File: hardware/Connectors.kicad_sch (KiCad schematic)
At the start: 4 parts, among them J2 Conn_02x20_Odd_Even, J3 M80-8420445, U1 AS222-35PN-933

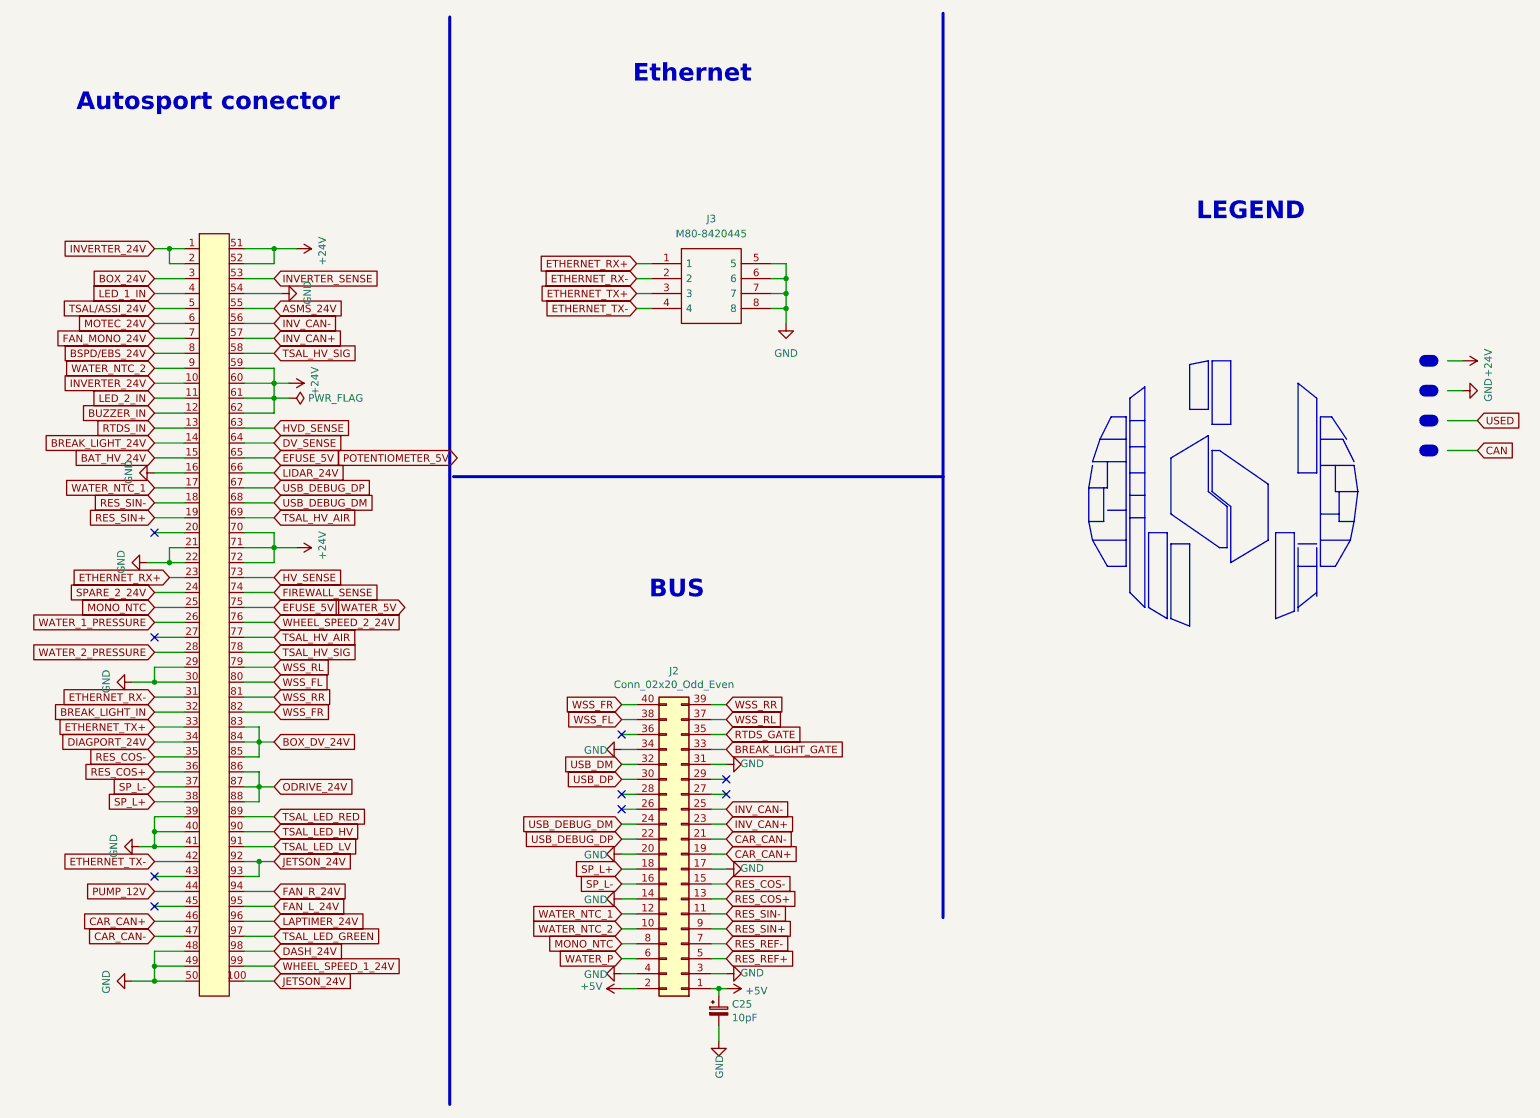
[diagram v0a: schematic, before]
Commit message: changed some footprints for clarity, and made some progress on board
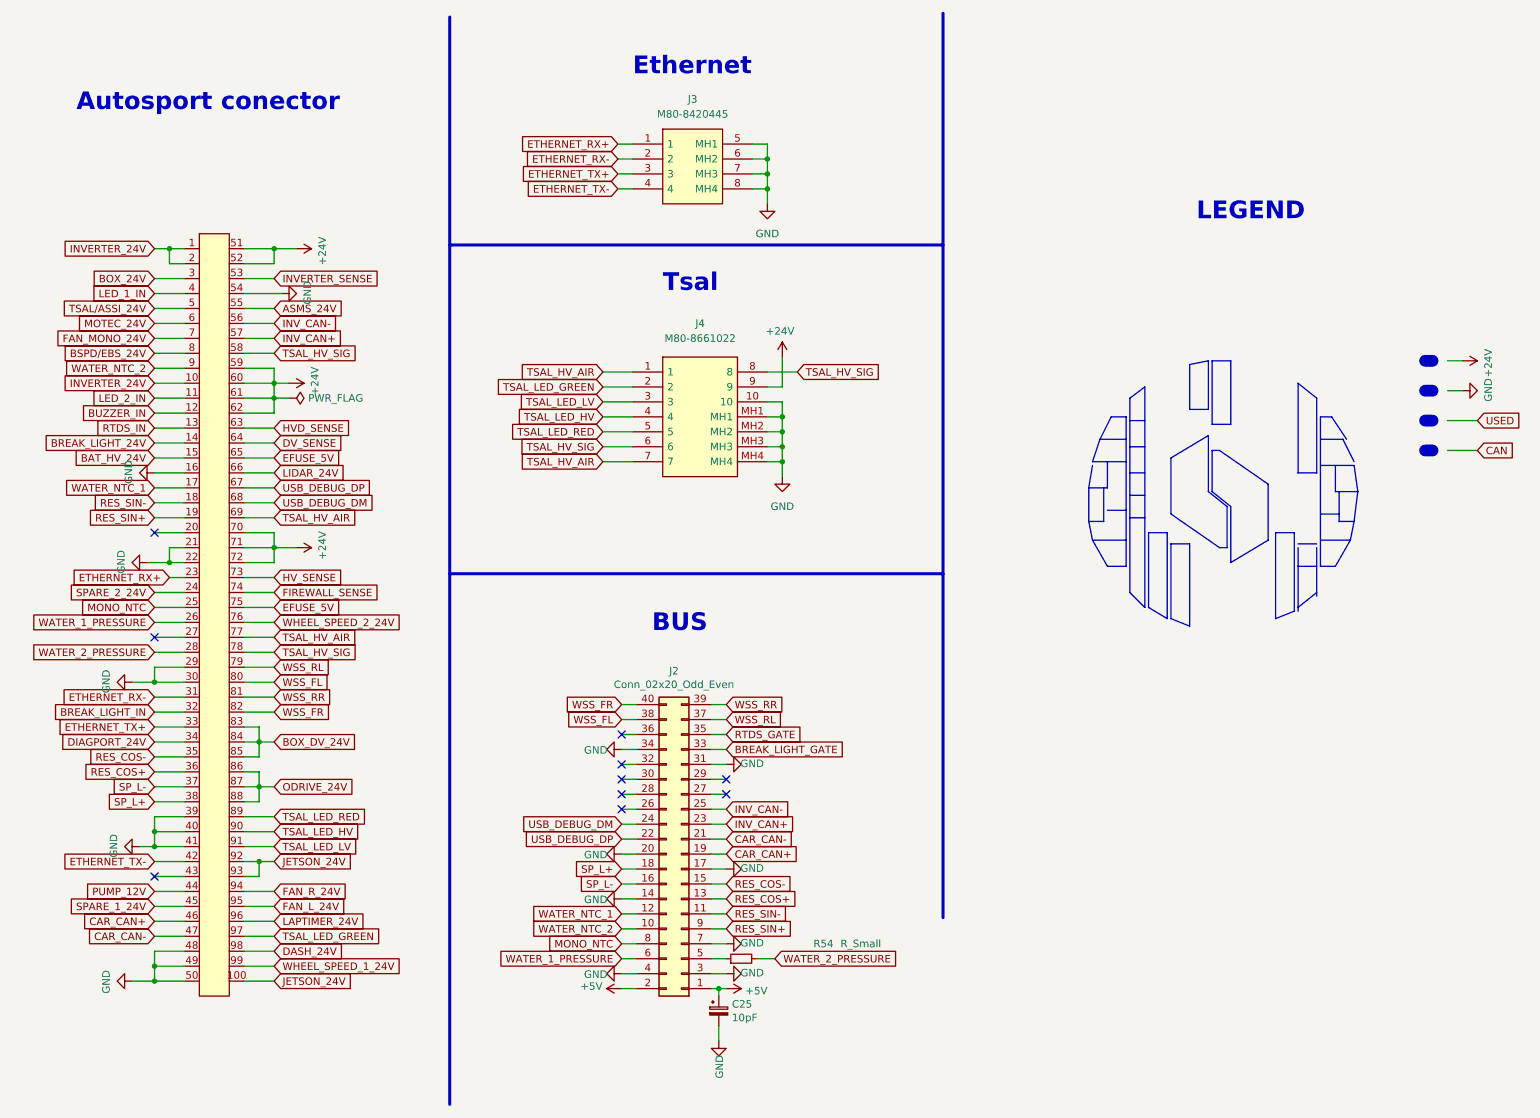
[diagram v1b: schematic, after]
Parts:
- added J4: M80-8661022, M80-8661022:M808661022, symbol M80-8661022:M80-8661022
- added R54: R_Small, Resistor_SMD:R_0603_1608Metric, symbol Device:R_Small
- J3: footprint M80-8420445 -> M80-8420445:M80-8420445
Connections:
- net RES_REF- is gone; now on net GND: J2.7 (Pin_7)
- net WATER_P is gone; now on net WATER_1_PRESSURE: J2.6 (Pin_6)
- net +24V: now also J4.9
- net GND: now also J4.10, J4.MH1, J4.MH2, J4.MH3, J4.MH4
- net TSAL_HV_AIR: now also J4.1, J4.7
- net TSAL_HV_SIG: now also J4.6, J4.8
- net TSAL_LED_GREEN: now also J4.2
- net TSAL_LED_HV: now also J4.4
- net TSAL_LED_LV: now also J4.3
- net TSAL_LED_RED: now also J4.5
- net WATER_2_PRESSURE: now also R54.2
- net SPARE_1_24V: now reaches U1.45
- net RES_REF+: no longer names the net of J2.5 (Pin_5)
- net RES_REF+: now also R54.1
- net USB_DM: no longer names the net of J2.32 (Pin_32)
- net USB_DP: no longer names the net of J2.30 (Pin_30)
- no-connect marks 9 -> 10
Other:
- note added: "Tsal"

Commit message: finished new wersion of the board
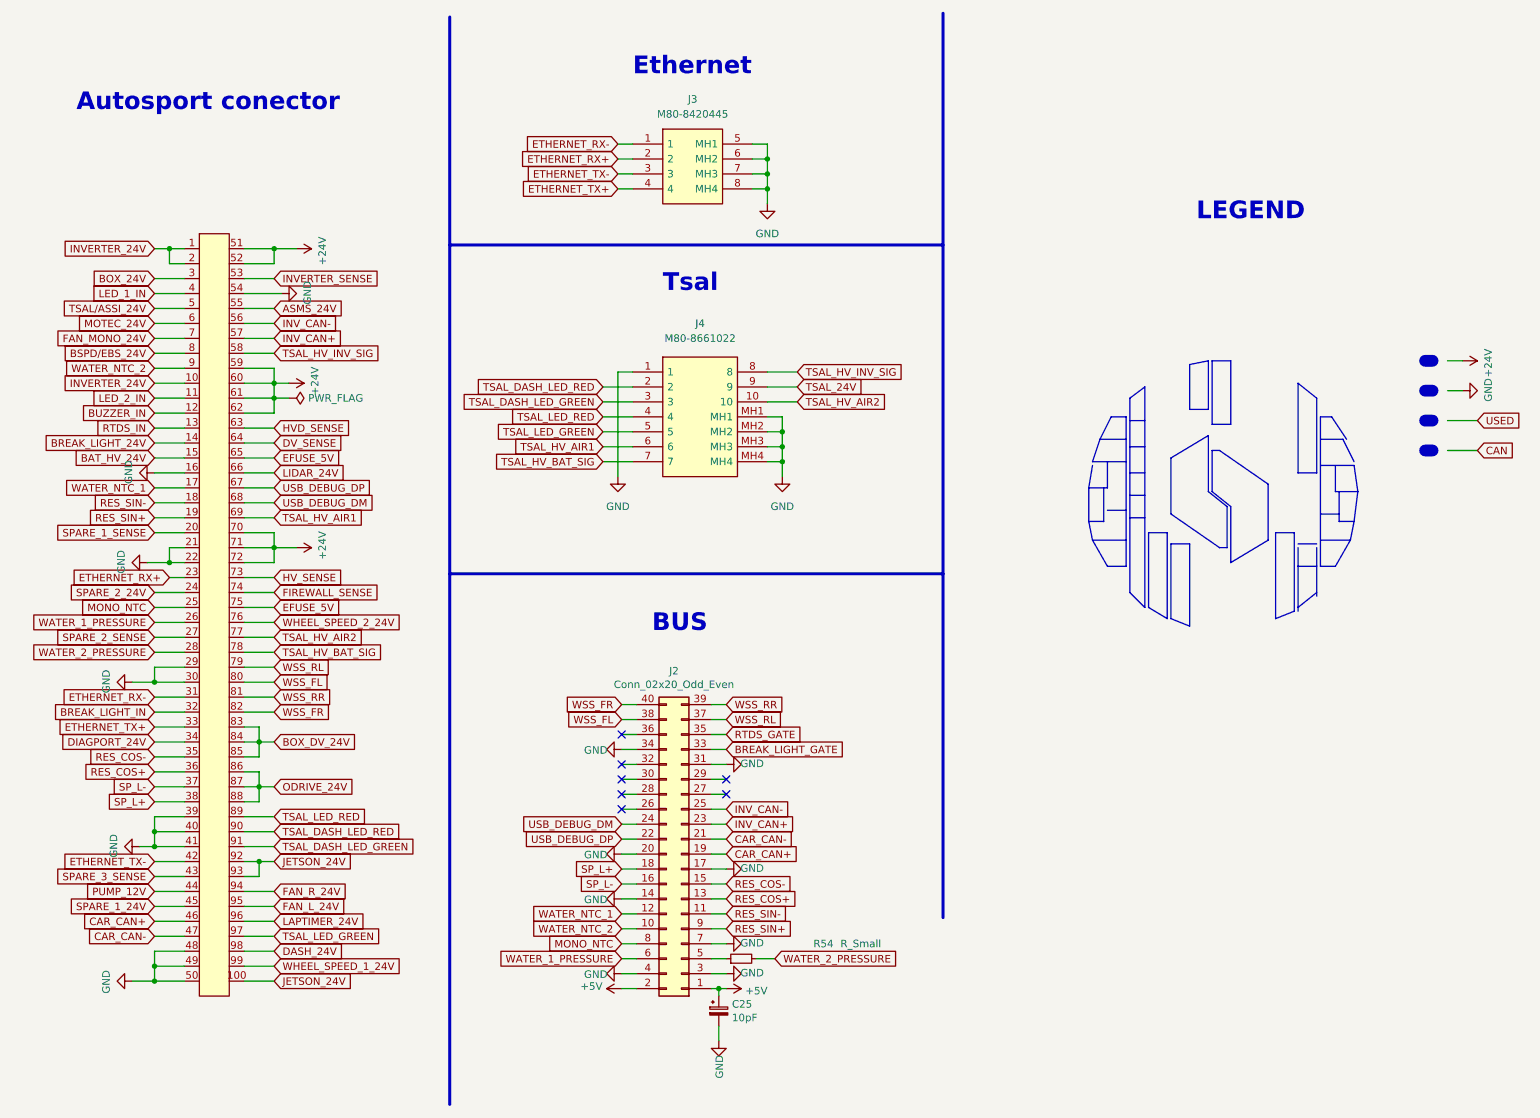
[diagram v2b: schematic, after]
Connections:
- net +24V: no longer J4.9
- net ETHERNET_RX+: now also J3.2; no longer J3.1
- net ETHERNET_RX-: now also J3.1; no longer J3.2
- net ETHERNET_TX+: now also J3.4; no longer J3.3
- net ETHERNET_TX-: now also J3.3; no longer J3.4
- net GND: now also J4.1; no longer J4.10
- net TSAL_LED_GREEN: now also J4.5; no longer J4.2
- net TSAL_LED_RED: now also J4.4; no longer J4.5
- net SPARE_1_SENSE: now reaches U1.20
- net SPARE_2_SENSE: now reaches U1.27
- net SPARE_3_SENSE: now reaches U1.43
- removed net TSAL_HV_AIR: J4.1, J4.7, U1.69, U1.77
- net TSAL_HV_SIG renamed TSAL_HV_INV_SIG
- net TSAL_HV_INV_SIG: no longer J4.6, U1.78
- net TSAL_LED_HV renamed TSAL_DASH_LED_RED
- net TSAL_DASH_LED_RED: now also J4.2; no longer J4.4
- net TSAL_LED_LV renamed TSAL_DASH_LED_GREEN
- new net TSAL_24V: J4.9
- new net TSAL_HV_AIR1: J4.6, U1.69
- new net TSAL_HV_AIR2: J4.10, U1.77
- new net TSAL_HV_BAT_SIG: J4.7, U1.78
- no-connect marks 10 -> 7
